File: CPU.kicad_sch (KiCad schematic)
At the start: 46 parts, among them Y1 X322524MKB4SI

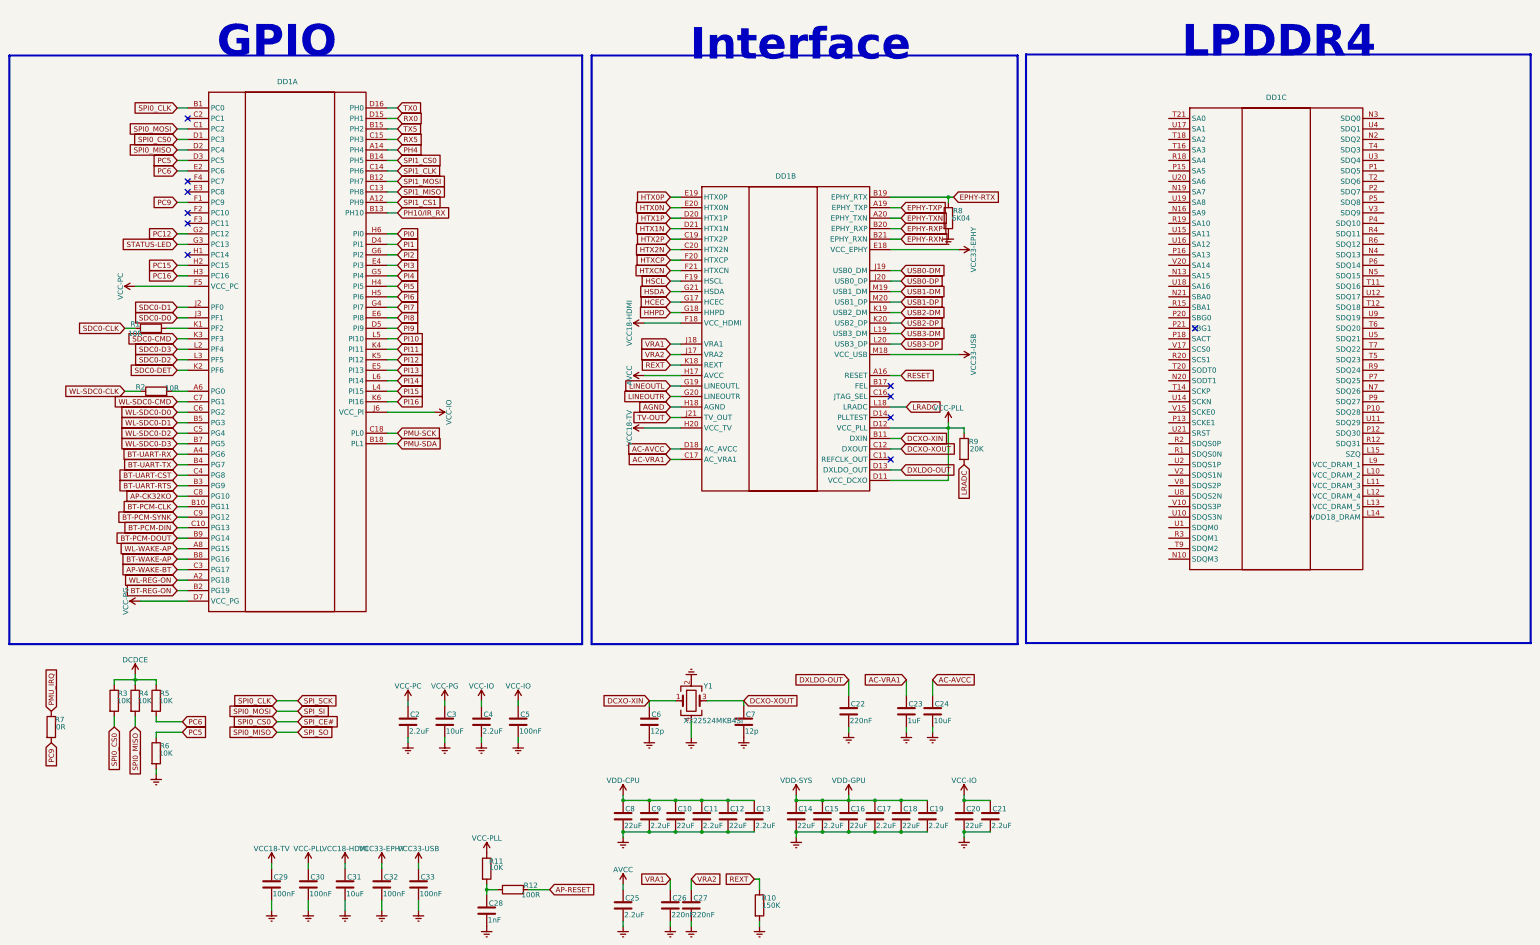
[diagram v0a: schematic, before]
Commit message: ddr
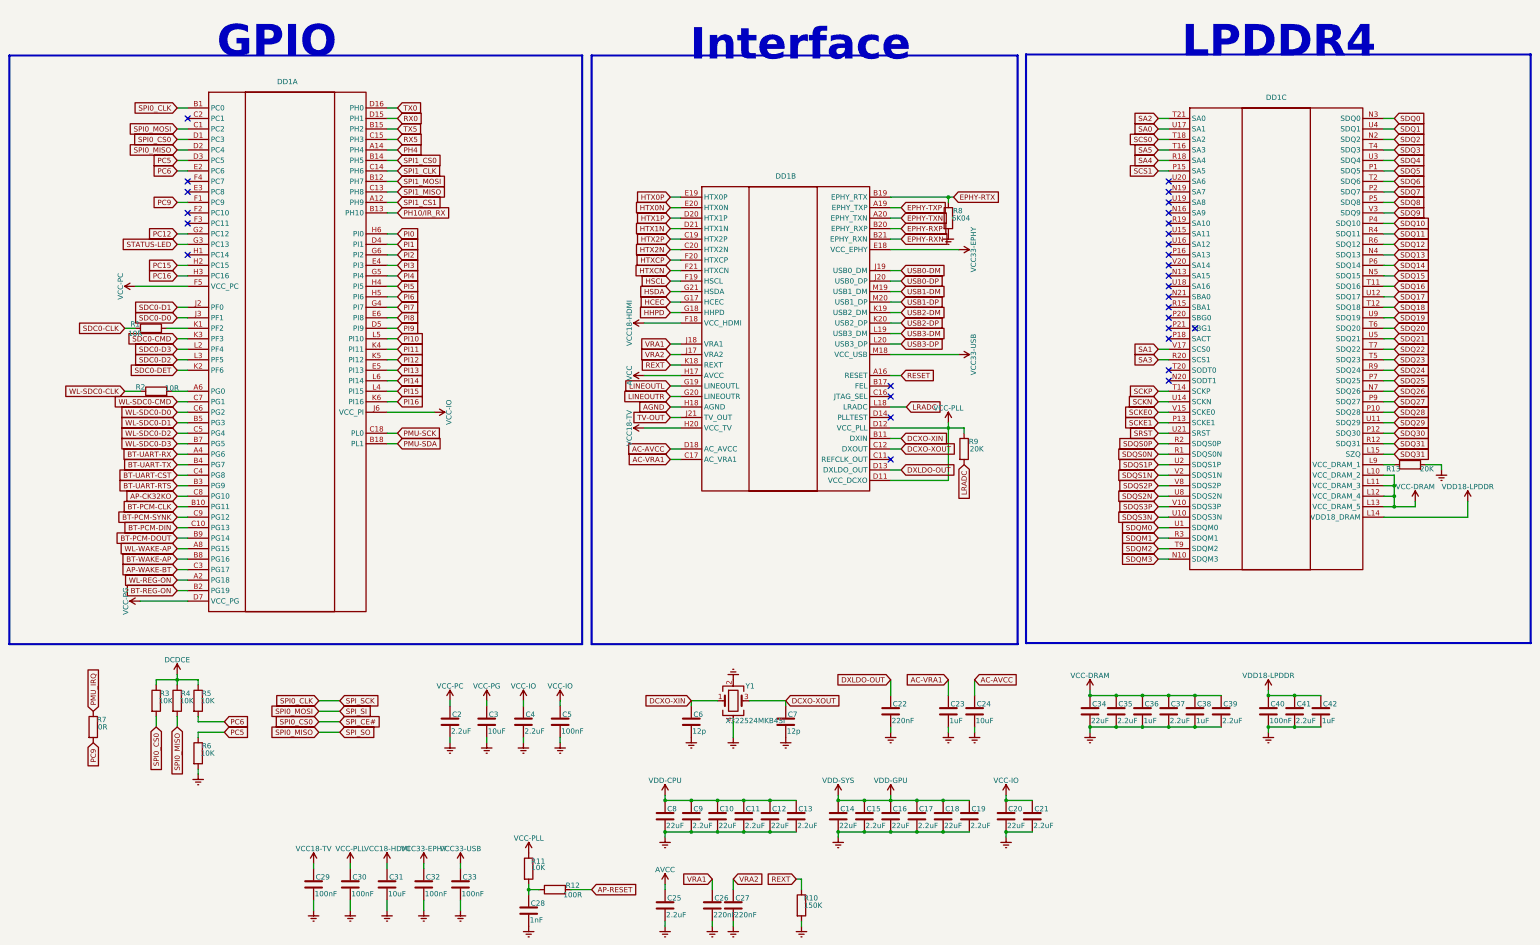
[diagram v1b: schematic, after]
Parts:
- added C34: 22uF, Capacitor_SMD:C_0402_1005Metric, symbol Device:C
- added C35, C37, C39, C41: 2.2uF, Capacitor_SMD:C_0402_1005Metric, symbol Device:C
- added C36, C38, C42: 1uF, Capacitor_SMD:C_0402_1005Metric, symbol Device:C
- added C40: 100nF, Capacitor_SMD:C_0402_1005Metric, symbol Device:C
- added R13: 20K, Resistor_SMD:R_0402_1005Metric, symbol Device:R
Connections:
- net Earth: now also C34.2, C35.2, C36.2, C37.2, C38.2, C39.2, C40.2, C41.2, C42.2, R13.2
- net VCC-DRAM: now reaches DD1.L10 (VCC_DRAM_2)
- net VCC-DRAM: now also DD1.L11 (VCC_DRAM_3), DD1.L12 (VCC_DRAM_4), DD1.L13 (VCC_DRAM_5), C34.1, C35.1, C36.1, C37.1, C38.1, C39.1
- net VDD18-LPDDR: now reaches DD1.L14 (VDD18_DRAM)
- net VDD18-LPDDR: now also C40.1, C41.1, C42.1
- net SDQ31: now reaches DD1.L15 (SZQ)
- net SDQ31: now also DD1.R12 (SDQ31)
- net at DD1.L9 (VCC_DRAM_1): now also R13.1
- net SDQM3: now reaches DD1.N10 (SDQM3)
- net SDQ2: now reaches DD1.N2 (SDQ2)
- net SDQ0: now reaches DD1.N3 (SDQ0)
- net SDQ13: now reaches DD1.N4 (SDQ13)
- net SDQ15: now reaches DD1.N5 (SDQ15)
- net SDQ26: now reaches DD1.N7 (SDQ26)
- net SDQ5: now reaches DD1.P1 (SDQ5)
- net SDQ28: now reaches DD1.P10 (SDQ28)
- net SDQ30: now reaches DD1.P12 (SDQ30)
- net SCKE1: now reaches DD1.P13 (SCKE1)
- net SCS1: now reaches DD1.P15 (SA5)
- net SDQ7: now reaches DD1.P2 (SDQ7)
- net SDQ10: now reaches DD1.P4 (SDQ10)
- net SDQ8: now reaches DD1.P5 (SDQ8)
- net SDQ14: now reaches DD1.P6 (SDQ14)
- net SDQ25: now reaches DD1.P7 (SDQ25)
- net SDQ27: now reaches DD1.P9 (SDQ27)
- net SDQS0N: now reaches DD1.R1 (SDQS0N)
- net SA4: now reaches DD1.R18 (SA4)
- net SDQS0P: now reaches DD1.R2 (SDQS0P)
- net SA3: now reaches DD1.R20 (SCS1)
- net SDQM1: now reaches DD1.R3 (SDQM1)
- net SDQ11: now reaches DD1.R4 (SDQ11)
- net SDQ12: now reaches DD1.R6 (SDQ12)
- net SDQ24: now reaches DD1.R9 (SDQ24)
- net SDQ16: now reaches DD1.T11 (SDQ16)
- net SDQ18: now reaches DD1.T12 (SDQ18)
- net SCKP: now reaches DD1.T14 (SCKP)
- net SA5: now reaches DD1.T16 (SA3)
- net SCS0: now reaches DD1.T18 (SA2)
- net SDQ6: now reaches DD1.T2 (SDQ6)
- net SA2: now reaches DD1.T21 (SA0)
- net SDQ3: now reaches DD1.T4 (SDQ3)
- net SDQ23: now reaches DD1.T5 (SDQ23)
- net SDQ20: now reaches DD1.T6 (SDQ20)
- net SDQ22: now reaches DD1.T7 (SDQ22)
- net SDQM2: now reaches DD1.T9 (SDQM2)
- net SDQM0: now reaches DD1.U1 (SDQM0)
- net SDQS3N: now reaches DD1.U10 (SDQS3N)
- net SDQ29: now reaches DD1.U11 (SDQ29)
- net SDQ17: now reaches DD1.U12 (SDQ17)
- net SCKN: now reaches DD1.U14 (SCKN)
- net SA0: now reaches DD1.U17 (SA1)
- net SDQS1P: now reaches DD1.U2 (SDQS1P)
- net SRST: now reaches DD1.U21 (SRST)
- net SDQ4: now reaches DD1.U3 (SDQ4)
- net SDQ1: now reaches DD1.U4 (SDQ1)
- net SDQ21: now reaches DD1.U5 (SDQ21)
- net SDQS2N: now reaches DD1.U8 (SDQS2N)
- net SDQ19: now reaches DD1.U9 (SDQ19)
- net SDQS3P: now reaches DD1.V10 (SDQS3P)
- net SCKE0: now reaches DD1.V15 (SCKE0)
- net SA1: now reaches DD1.V17 (SCS0)
- net SDQS1N: now reaches DD1.V2 (SDQS1N)
- net SDQ9: now reaches DD1.V3 (SDQ9)
- net SDQS2P: now reaches DD1.V8 (SDQS2P)
- no-connect marks 11 -> 29
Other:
- moved on the sheet: C10, C11, C12, C13, C14, C15, C16, C17, C18, C19, C2, C20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
